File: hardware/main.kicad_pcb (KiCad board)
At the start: 2 copper layers, 100 x 72.4 mm, 16 parts, among them J2 M300-MV10345M1, J4 ScrewTerminal, J5 ScrewTerminal, J6 ScrewTerminal, K2 ADW11

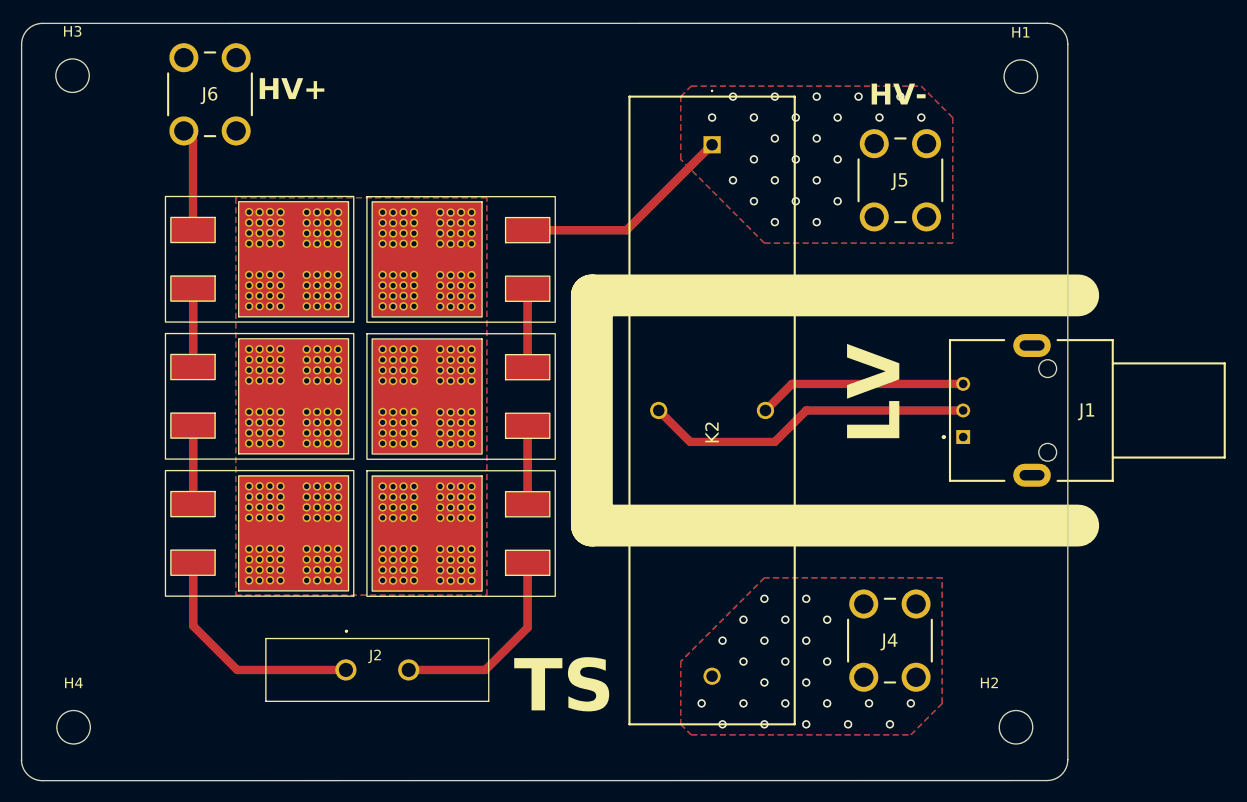
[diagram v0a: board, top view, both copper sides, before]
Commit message: Zmniejszona
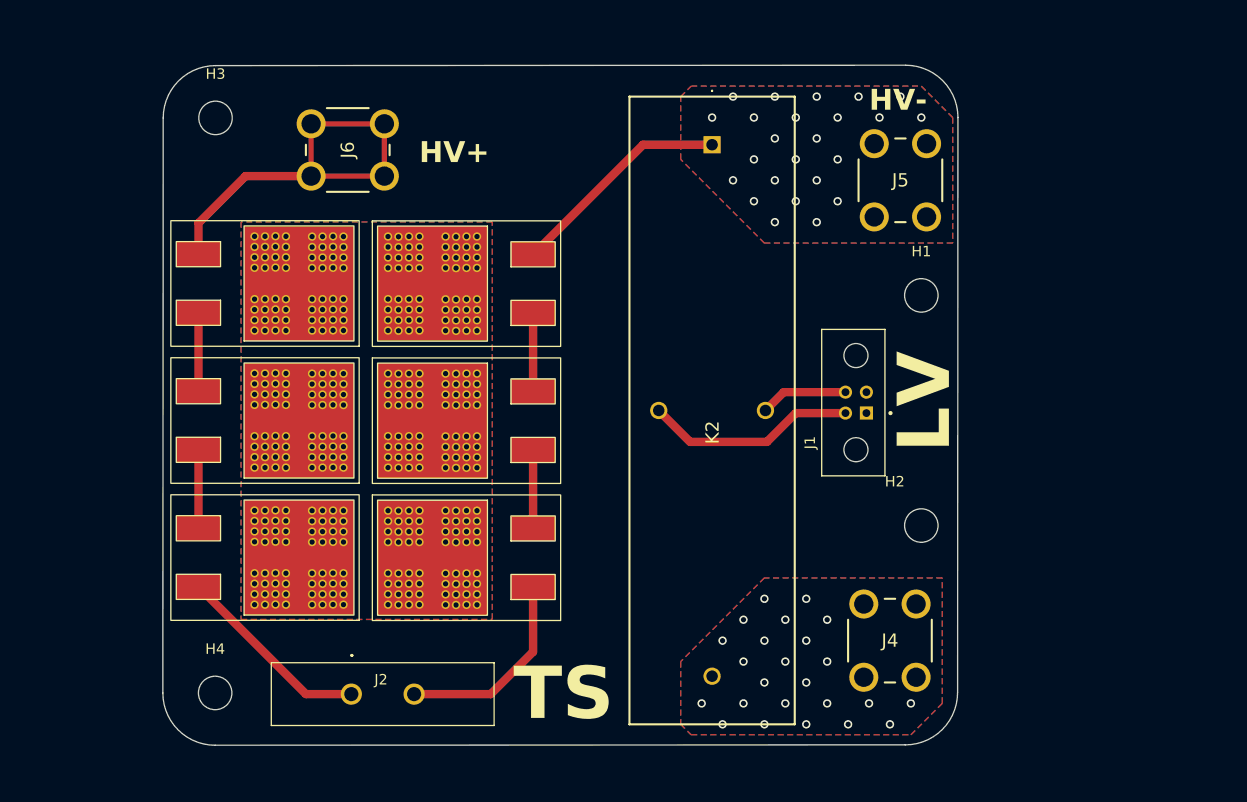
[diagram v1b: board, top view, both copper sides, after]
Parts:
- J1: value ~ -> Conn_01x04; footprint d369-g33-xx:D369-G33-XX -> Harwin_m80:HARWIN_M80-5100442
- moved H1 23.0 mm to (193.0, 72.0)
- moved H2 21.3 mm to (193.0, 94.0)
- moved H3 14.2 mm to (125.5, 55.0)
- moved H4 13.9 mm to (125.5, 110.0)
- moved J1 10.8 mm to (186.8, 82.2), turned to 90 degrees
- moved J6 9.55 mm to (134.7, 55.6), turned to -90 degrees
- moved R4 2.37 mm to (151.5, 97.1)
- moved R6 2.37 mm to (151.5, 70.9)
- moved J2 2.37 mm to (138.5, 110.1)
- moved R1 2.37 mm to (128.3, 70.9)
- moved R3 2.37 mm to (128.3, 97.1)
- moved R5 2.37 mm to (151.5, 84.0)
- moved R2 2.37 mm to (128.3, 84.0)
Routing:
- net HV+: track 9.82 -> 39.7 mm
- net GND: track 20.0 -> 8.37 mm
- net SD+: track 31.6 -> 20.2 mm
- net TSMP+: track 22.4 -> 18.9 mm
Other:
- board size 100 x 72.4 mm -> 76 x 65 mm
